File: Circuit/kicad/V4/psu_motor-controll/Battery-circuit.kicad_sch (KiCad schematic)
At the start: 13 parts, among them J3 Charge, Q2 IRFR7546TRPBF, Q3 IRFR7546TRPBF

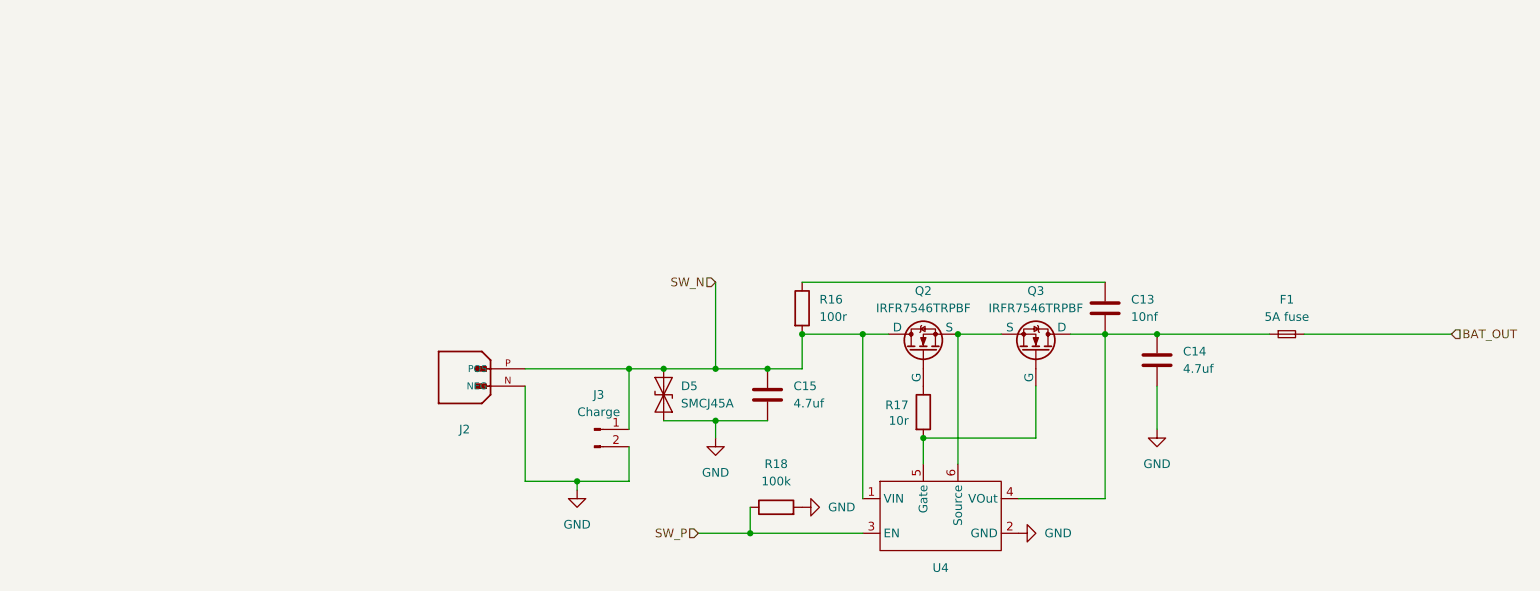
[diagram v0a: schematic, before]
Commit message: PSU FINISH BOARD NO DRC,ERC,DFM ERRORS
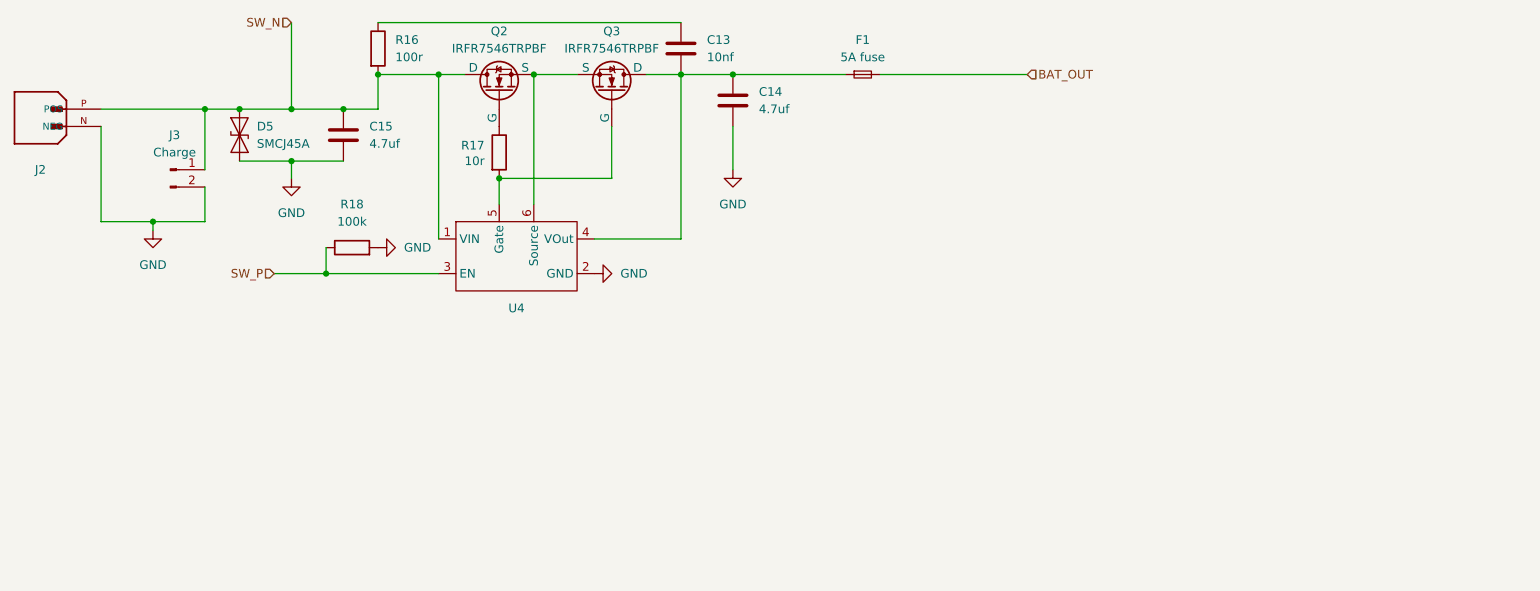
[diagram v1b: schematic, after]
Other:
- moved on the sheet: C13, C14, C15, D5, F1, J2, J3, Q2, Q3, R16, R17, R18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
